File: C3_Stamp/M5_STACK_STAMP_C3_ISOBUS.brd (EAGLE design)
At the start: 20.3 x 22.9 mm, 3 parts, among them J1 61300811121, J2 61300611121

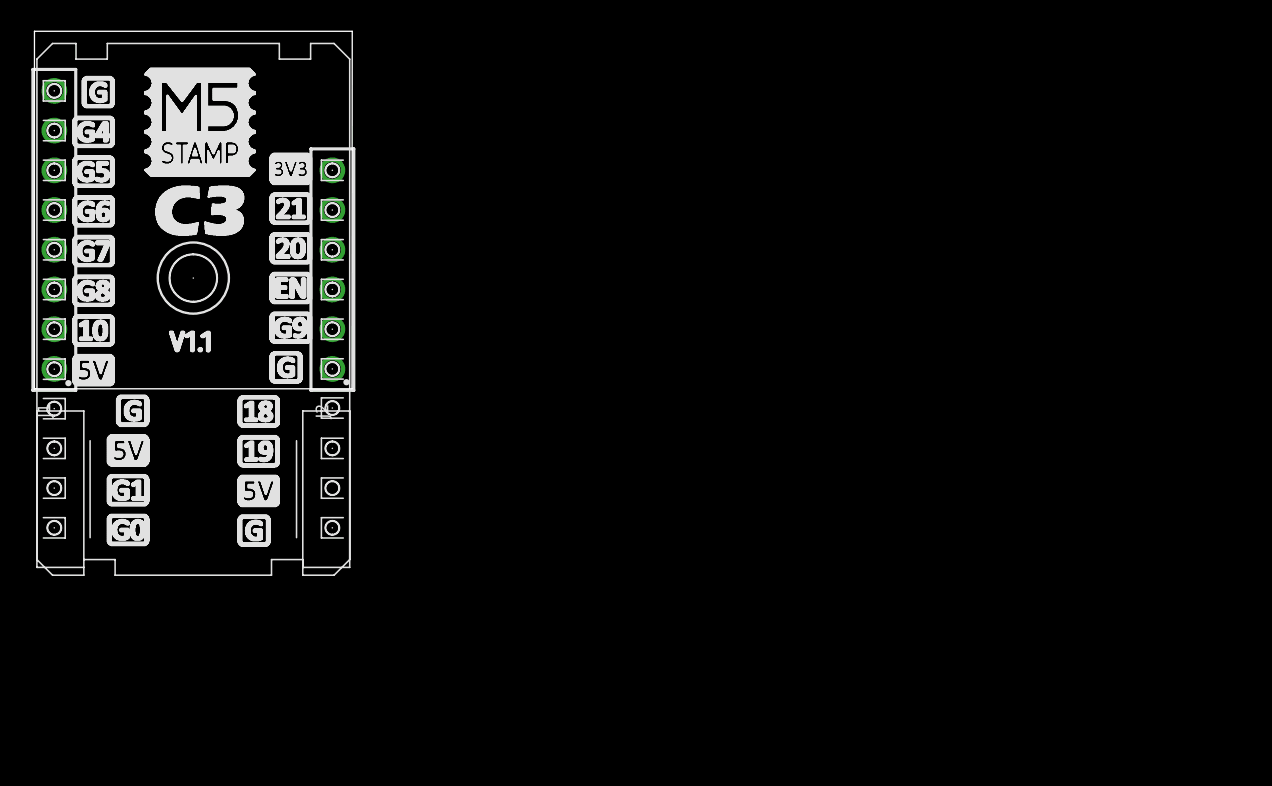
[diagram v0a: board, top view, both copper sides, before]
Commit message: ..
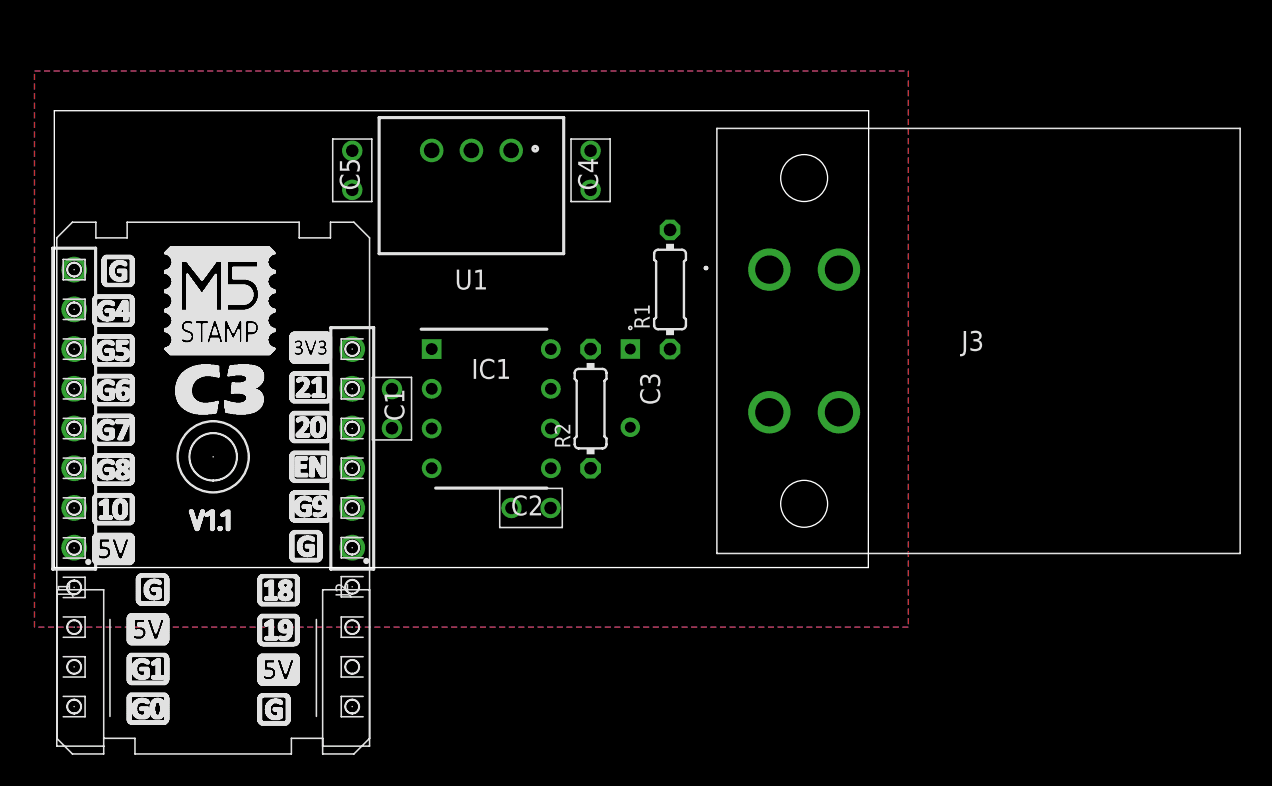
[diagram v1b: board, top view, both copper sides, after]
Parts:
- added C1, C2, C4, C5: FG18X7R1H104KNT06, FG18X7R1H104KNT06-pcb-part-libraries:FG18C0G1H101JNT06
- added C3: FG28X7R1H473KNT06, FG28X7R1H473KNT06-pcb-part-libraries:FG28
- added IC1: MCP2562-E_P, MCP2562-E_P-pcb-part-libraries:DIP781W56P254L950H533Q8N
- added J3: DTF13-4P, DTF13-4P-pcb-part-libraries:DTF134P
- added R1, R2: (no value), resistor:0204/7
- added U1: (no value), Wurth_Step Down Converter_MagI³C-FDSM:MAGI³C-FDSM_173XXXX42
- moved J1 11.5 mm to (2.54, 11.4)
- moved J2 11.5 mm to (20.3, 8.89)
- moved U$1 11.5 mm to (2.54, 20.3)
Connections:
- new net +12V: C4.2, J3.1, U1.1
- new net +3V3: C2.2, IC1.5, J2.6
- new net +5V: C1.2, C5.2, IC1.3, J1.8, U1.3
- new net CAN_N: IC1.6, J3.4, R2.1
- new net CAN_P: IC1.7, J3.2, R1.2
- new net EN: J2.3
- new net G10: J1.7
- new net G20: IC1.4, J2.4
- new net G21: IC1.1, J2.5
- new net G4: J1.2
- new net G5: J1.3
- new net G6: J1.4
- new net G7: J1.5
- new net G8: J1.6
- new net G9: J2.2
- new net GND: C1.1, C2.1, C3.2, C4.1, C5.1, IC1.2, IC1.8, J1.1, J2.1, J3.3, U1.2
- new net N$1: C3.1, R1.1, R2.2
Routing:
- added copper zone on layer 1, net GND
- added copper zone on layer 16, net GND
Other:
- board size 20.3 x 22.9 mm -> 52.1 x 29.2 mm

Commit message: Order !
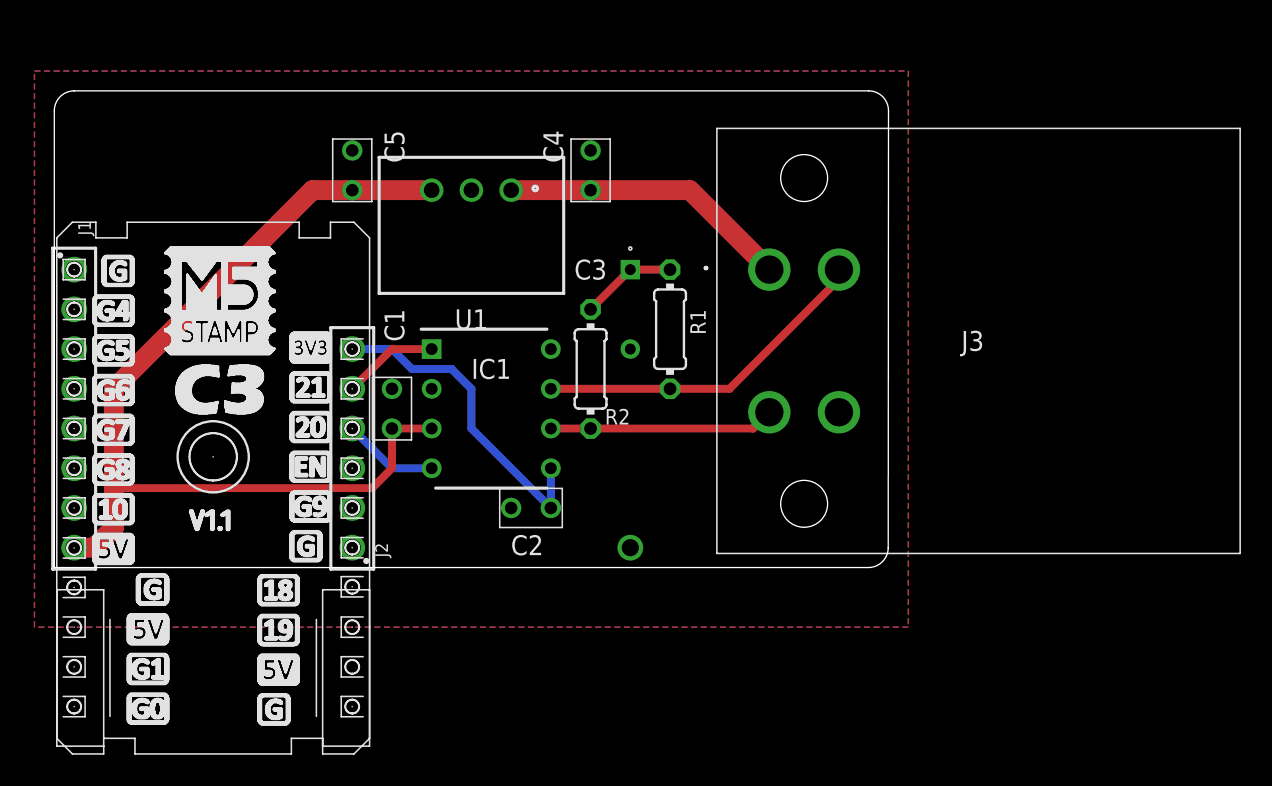
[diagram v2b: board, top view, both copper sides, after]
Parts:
- moved C3 5.08 mm to (38.1, 20.3)
- moved U1 2.54 mm to (27.9, 25.4)
- moved R2 2.54 mm to (35.6, 14.0)
- moved R1 2.54 mm to (40.6, 16.5), turned to 270 degrees
- turned C4 to 270 degrees
- turned C5 to 270 degrees
- turned J1 to 270 degrees
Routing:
- net +5V: track 0.00 -> 60.9 mm
- net CAN_P: track 0.00 -> 21.9 mm
- net +3V3: track 0.00 -> 20.9 mm
- net +12V: track 0.00 -> 18.6 mm
- net CAN_N: track 0.00 -> 14.4 mm
- net G21: track 0.00 -> 6.13 mm
- net G20: track 0.00 -> 6.13 mm
- net N$1: track 0.00 -> 6.13 mm
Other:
- board size 52.1 x 29.2 mm -> 53.3 x 30.5 mm
